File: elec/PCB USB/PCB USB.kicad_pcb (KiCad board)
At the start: 2 copper layers, 91 x 38 mm, 99 parts, among them J201 USB_C_PICO, J402 USB_C_Receptacle_USB2.0_14P, J403 USB_A, J404 USB_C_Receptacle_USB2.0_14P, J405 USB_A, J501 Conn_I2C_Écran, P1 USB_C_Plug_USB2.0, Q301 AO3401A, Q401 AO3401A, SW201 SW_BOOTSEL, SW202 SW_RESET, SW501 RotaryEncoder_Switch, U201 SRV05-4, U202 RP2350B-QFN80, U203 W25Q128JVPIQ, U301 AP7361C-33E, U401 SRV05-4, Y201 CM4012M00012001, Y401 12MHz

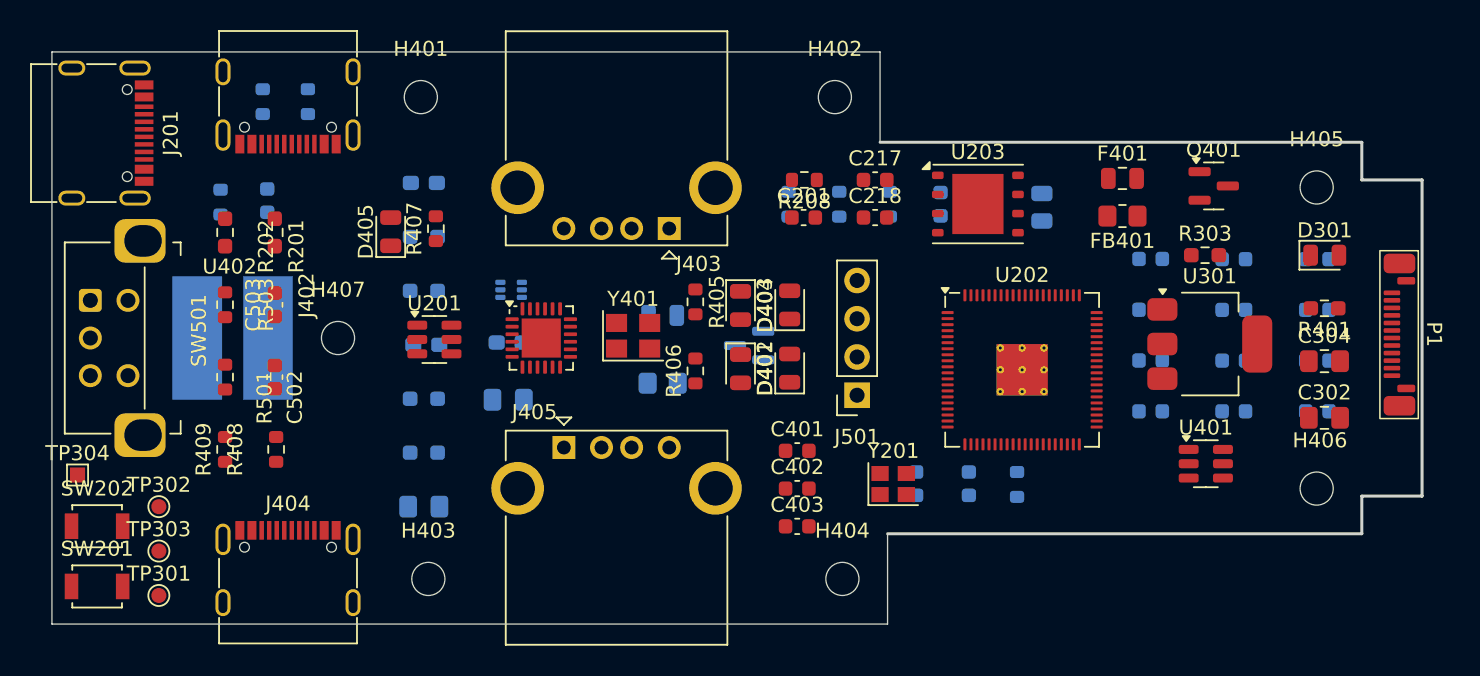
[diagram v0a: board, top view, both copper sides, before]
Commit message: push pcb
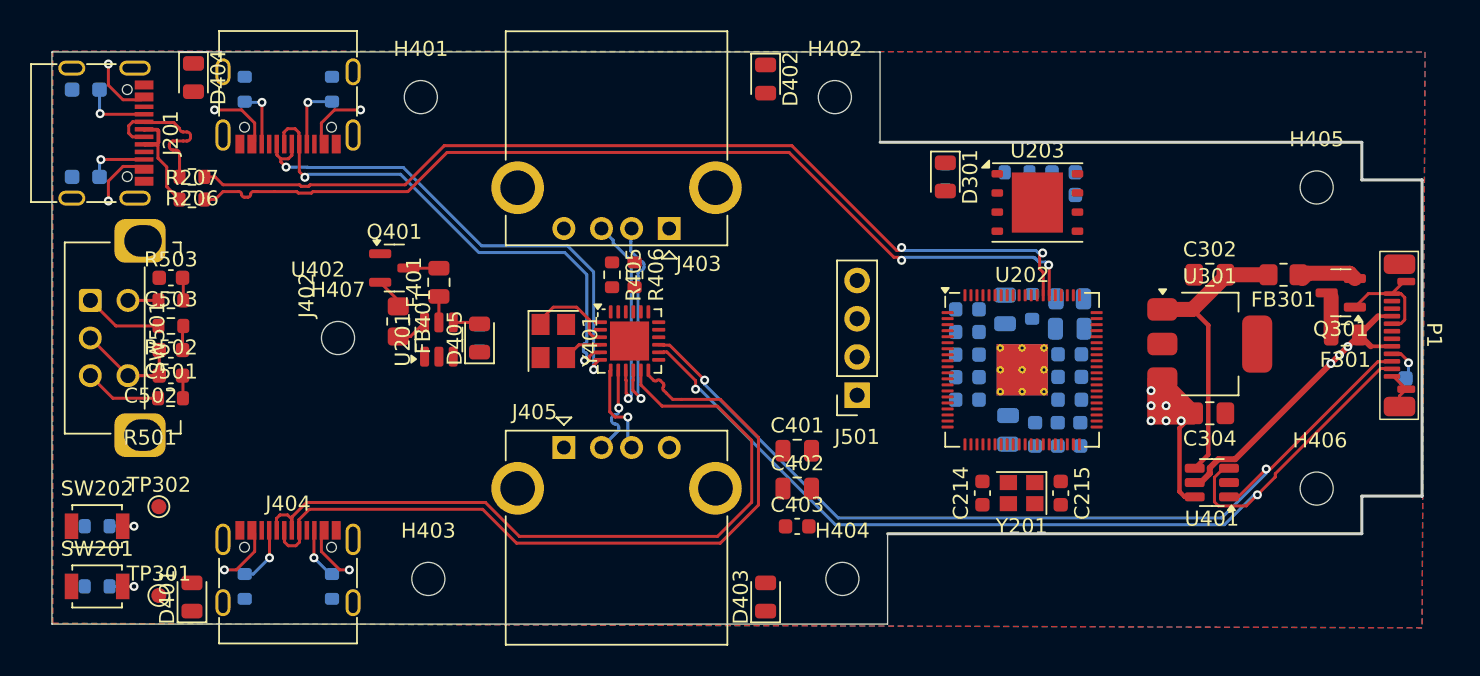
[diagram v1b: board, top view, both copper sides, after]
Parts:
- removed C301: 10µF, Capacitor_SMD:C_0805_2012Metric_Pad1.18x1.45mm_HandSolder
- removed C303, C307: 0.1µF, Capacitor_SMD:C_0603_1608Metric_Pad1.08x0.95mm_HandSolder
- removed C305: 33pF, Capacitor_SMD:C_0603_1608Metric_Pad1.08x0.95mm_HandSolder
- removed C306: 22µF, Capacitor_SMD:C_0805_2012Metric_Pad1.18x1.45mm_HandSolder
- removed L301: 2.2uH 13.2mOhm, Inductor_SMD:L_TDK_VLP8040
- removed R301: 100k, Resistor_SMD:R_0603_1608Metric_Pad0.98x0.95mm_HandSolder
- removed R302: 17.4k, Resistor_SMD:R_0603_1608Metric_Pad0.98x0.95mm_HandSolder
- removed R304: 220k, Resistor_SMD:R_0603_1608Metric_Pad0.98x0.95mm_HandSolder
- removed R305: 30k, Resistor_SMD:R_0603_1608Metric_Pad0.98x0.95mm_HandSolder
- removed TP303: TP_5V, TestPoint:TestPoint_Pad_D1.0mm
- removed TP304: TP_GND, TestPoint:TestPoint_Pad_1.0x1.0mm
- removed U302: ~, Package_TO_SOT_SMD:SOT-563
- C201, C217, C218, R201, R202, R208, R303, R401, R407, R408, R409: moved to B.Cu
- C209, C213, C216, C401, C402: footprint Capacitor_SMD:C_0603_1608Metric -> Capacitor_SMD:C_0805_2012Metric
- C214, C215, C501, F301, FB301, Q301, R206, R207, R502: moved to F.Cu
- moved R203 61.2 mm to (87.5, 110.5), turned to 0 degrees
- moved Q401 54.7 mm to (107.2, 93.3)
- moved R204 52.5 mm to (87.5, 114.5), turned to 0 degrees
- moved FB401 48.6 mm to (107.5, 96.9), turned to -90 degrees
- moved R207 46.4 mm to (93.8, 88.8), turned to 0 degrees
- moved F401 45.9 mm to (110.2, 94.3), turned to 90 degrees
- moved F301 45.4 mm to (170.4, 97.8), turned to 180 degrees
- moved R206 43.0 mm to (93.8, 87.3), turned to 180 degrees
- moved FB301 41.9 mm to (166.3, 93.8)
- moved D401 39.5 mm to (93.8, 115.2), turned to 90 degrees
- moved Q301 39.5 mm to (170.1, 95.0)
- moved D404 39.4 mm to (93.9, 80.7)
- moved D301 25.7 mm to (143.8, 87.3), turned to -90 degrees
- moved C209 23.5 mm to (148.0, 104.1), turned to 90 degrees
- moved D403 19.5 mm to (131.9, 115.2)
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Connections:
- FB301 pad 2: +5V_PROTECT -> +5V
- TP301 pad 1: +5V_PROTECT -> +5V
- Y401 pad 2: Net-(U402-X_{IN}) -> (no net)
- Y401 pad 3: (no net) -> Net-(U402-X_{IN})
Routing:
- net /USB_HUB/D-: track 0.00 -> 64.3 mm, vias 0 -> 2
- net /MCU/D-: track 0.00 -> 63.2 mm, vias 0 -> 2
- net /MCU/D+: track 0.00 -> 63.1 mm, vias 0 -> 2
- net /USB_HUB/D+: track 0.00 -> 61.3 mm, vias 0 -> 2
- net VBUS: track 0.00 -> 60.4 mm, vias 0 -> 9
- net /USB_HUB/USBC_1_D+: track 0.00 -> 50.4 mm
- net /USB_HUB/USBC_1_D-: track 0.00 -> 50.4 mm
- net /USB_HUB/USBC_2_D+: track 0.00 -> 34.1 mm, vias 0 -> 2
- net /USB_HUB/USBC_2_D-: track 0.00 -> 34.1 mm, vias 0 -> 2
- net +5V: track 0.00 -> 21.6 mm
- net GND: track 0.00 -> 17.5 mm
- net /USB_HUB/USBA_2_D-: track 0.00 -> 14.1 mm, vias 0 -> 1
- net /USB_HUB/USBA_2_D+: track 0.00 -> 14.1 mm, vias 0 -> 1
- net +3V3: track 0.00 -> 11.7 mm, vias 0 -> 6
- net /MCU/USB_PICO_D+: track 0.00 -> 10.8 mm
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- added copper zone on In2.Cu, net +3V3
- added copper zone on B.Cu, net GND
- added copper zone on F.Cu, net GND
- added copper zone on In1.Cu, net GND
- added copper zone on In2.Cu, net VBUS
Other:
- copper layers 2 -> 4

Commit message: oh shit game de volley
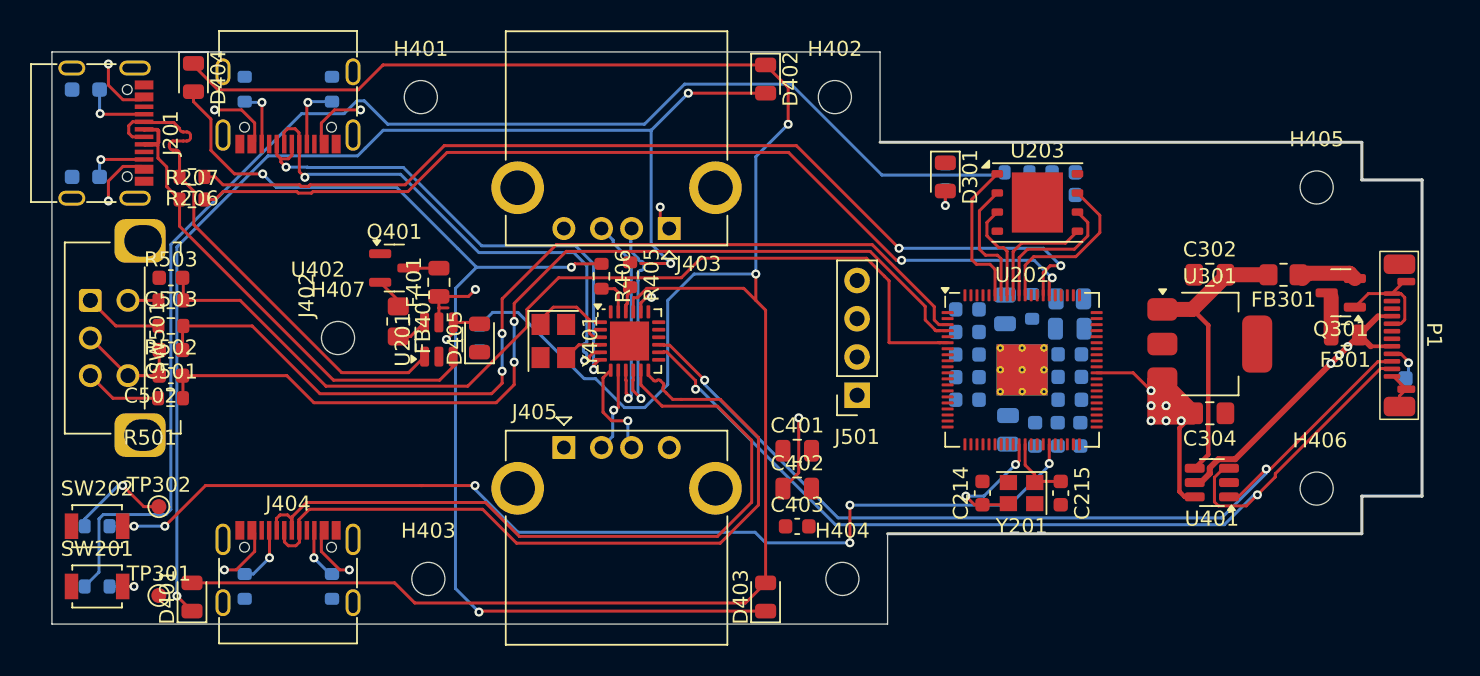
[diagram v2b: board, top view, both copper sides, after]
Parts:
- moved R406 2.20 mm to (121.0, 93.9)
- moved R405 1.20 mm to (122.9, 93.8)
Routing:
- net VBUS: track 60.4 -> 248.9 mm, vias 9 -> 11
- net Net-(D401-A): track 0.00 -> 152.9 mm, vias 0 -> 2
- net +3V3: track 11.7 -> 113.6 mm, vias 6 -> 10
- net /MCU/~{QSPI_CS_{0}}: track 0.00 -> 101.1 mm
- net Net-(D401-K): track 0.00 -> 79.4 mm, vias 0 -> 3
- net Net-(D403-K): track 0.00 -> 76.8 mm, vias 0 -> 3
- net /MCU/~{RESET}: track 2.38 -> 71.1 mm, vias 1 -> 6
- net /MCU/GPIO6: track 1.62 -> 64.3 mm, vias 0 -> 2
- net /MCU/GPIO7: track 1.51 -> 63.8 mm, vias 0 -> 2
- net /MCU/GPIO8: track 1.52 -> 63.7 mm
- net /MCU/USB_PICO_D+: track 10.8 -> 36.0 mm
- net /MCU/USB_PICO_D-: track 10.6 -> 34.1 mm
- net /MCU/QSPI_SD3: track 0.00 -> 11.1 mm
- net /MCU/QSPI_SCLK: track 0.00 -> 9.53 mm
- net Net-(U202-XIN): track 0.00 -> 8.98 mm, vias 0 -> 2
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- removed copper zone on B.Cu, net GND
- removed copper zone on F.Cu, net GND
- removed copper zone on In1.Cu, net GND
